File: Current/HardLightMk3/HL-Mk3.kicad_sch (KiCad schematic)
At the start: 225 parts, among them J0 USB, K1 Keyswitch, K10 Keyswitch, K11 Keyswitch, K12 Keyswitch, K13 Keyswitch, K14 Keyswitch, K15 Keyswitch, K16 Keyswitch, K17 Keyswitch, K18 Keyswitch, K19 Keyswitch, K2 Keyswitch, K20 Keyswitch, K21 Keyswitch, K22 Keyswitch, K23 Keyswitch, K24 Keyswitch, K25 Keyswitch, K26 Keyswitch, K27 Keyswitch, K28 Keyswitch, K29 Keyswitch, K3 Keyswitch, K30 Keyswitch, K31 Keyswitch, K32 Keyswitch, K33 Keyswitch, K34 Keyswitch, K35 Keyswitch, K36 Keyswitch, K37 Keyswitch, K38 Keyswitch, K39 Keyswitch, K4 Keyswitch, K40 Keyswitch, K41 Keyswitch, K42 Keyswitch, K43 Keyswitch, K44 Keyswitch, K45 Keyswitch, K46 Keyswitch, K47 Keyswitch, K48 Keyswitch, K49 Keyswitch, K5 Keyswitch, K50 Keyswitch, K51 Keyswitch, K52 Keyswitch, K53 Keyswitch, K54 Keyswitch, K55 Keyswitch, K56 Keyswitch, K57 Keyswitch, K58 Keyswitch, K59 Keyswitch, K6 Keyswitch, K60 Keyswitch, K61 Keyswitch, K62 Keyswitch, K63 Keyswitch, K64 Keyswitch, K7 Keyswitch, K8 Keyswitch, K9 Keyswitch, U0 STM32F411CEU6, U1 LDO-3.3, Y0 8MHz

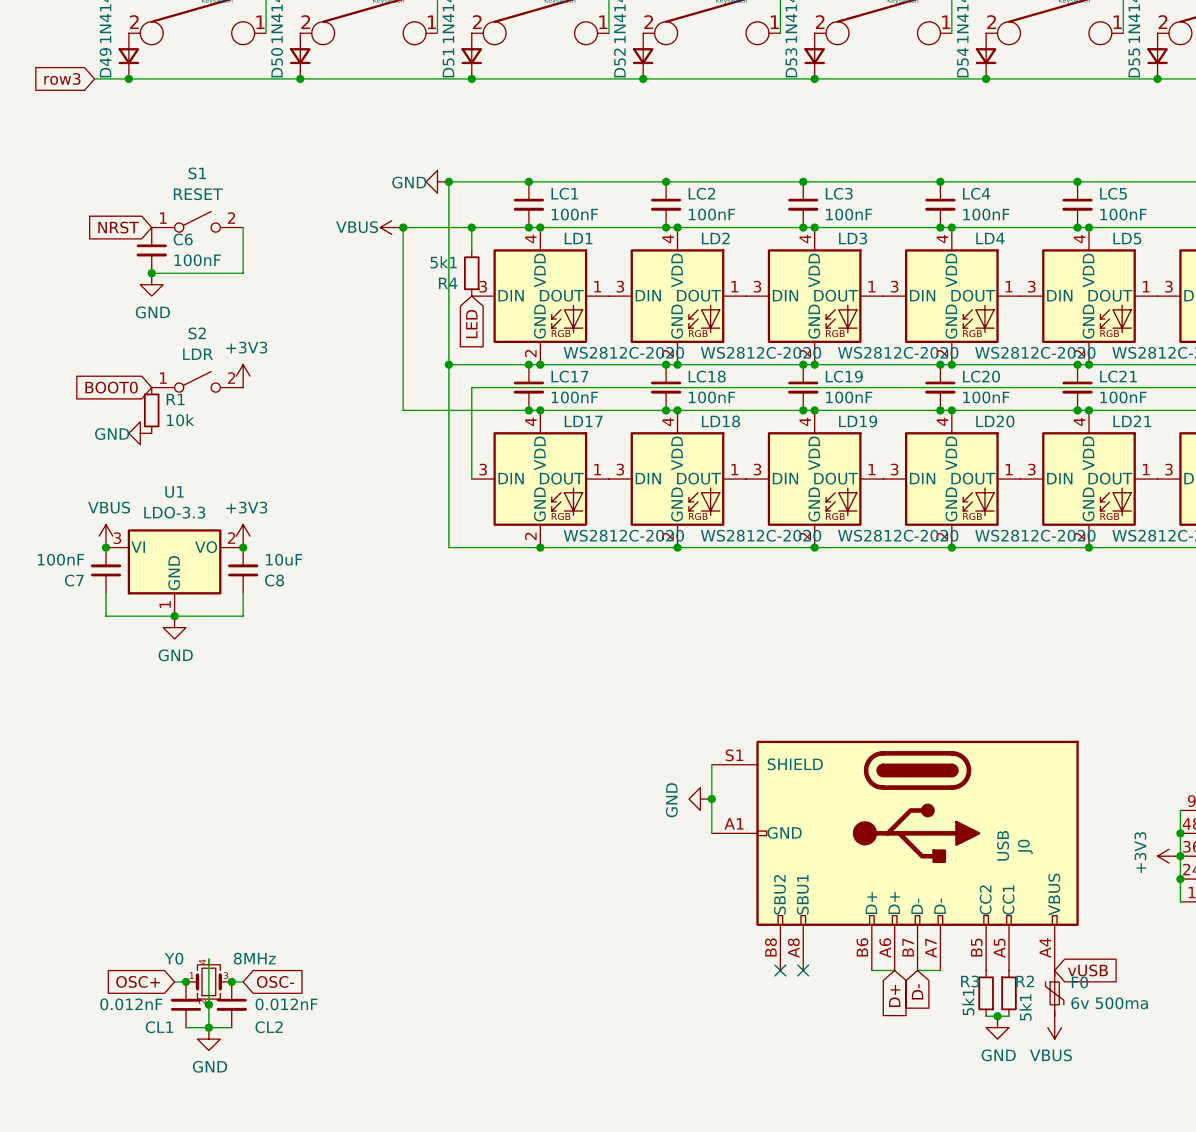
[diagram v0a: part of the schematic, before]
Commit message: Hard Light Micro 5, Borealis, 2T, SB
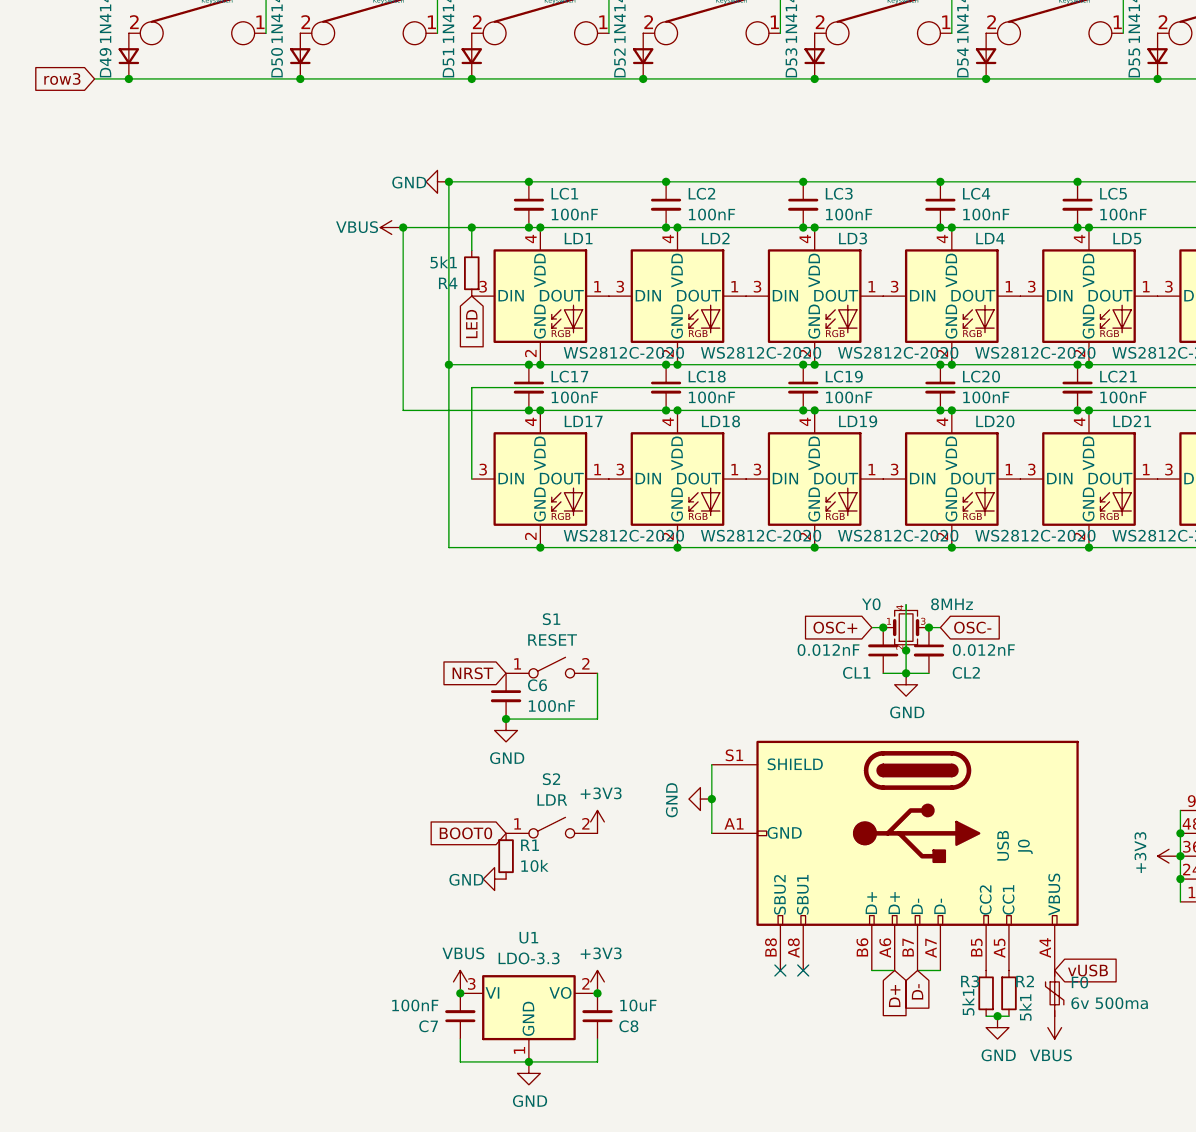
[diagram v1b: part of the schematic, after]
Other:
- moved on the sheet: C6, C7, C8, CL1, CL2, R1, S1, S2, U1, Y0
